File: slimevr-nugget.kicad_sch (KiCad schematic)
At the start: 56 parts, among them U1 nRF52840-QFXX, U3 XC6220B331MR, U4 LSM6DSV, U5 1532H, U6 QMC6309, U7 BQ24073RGT, Y1 32MHz

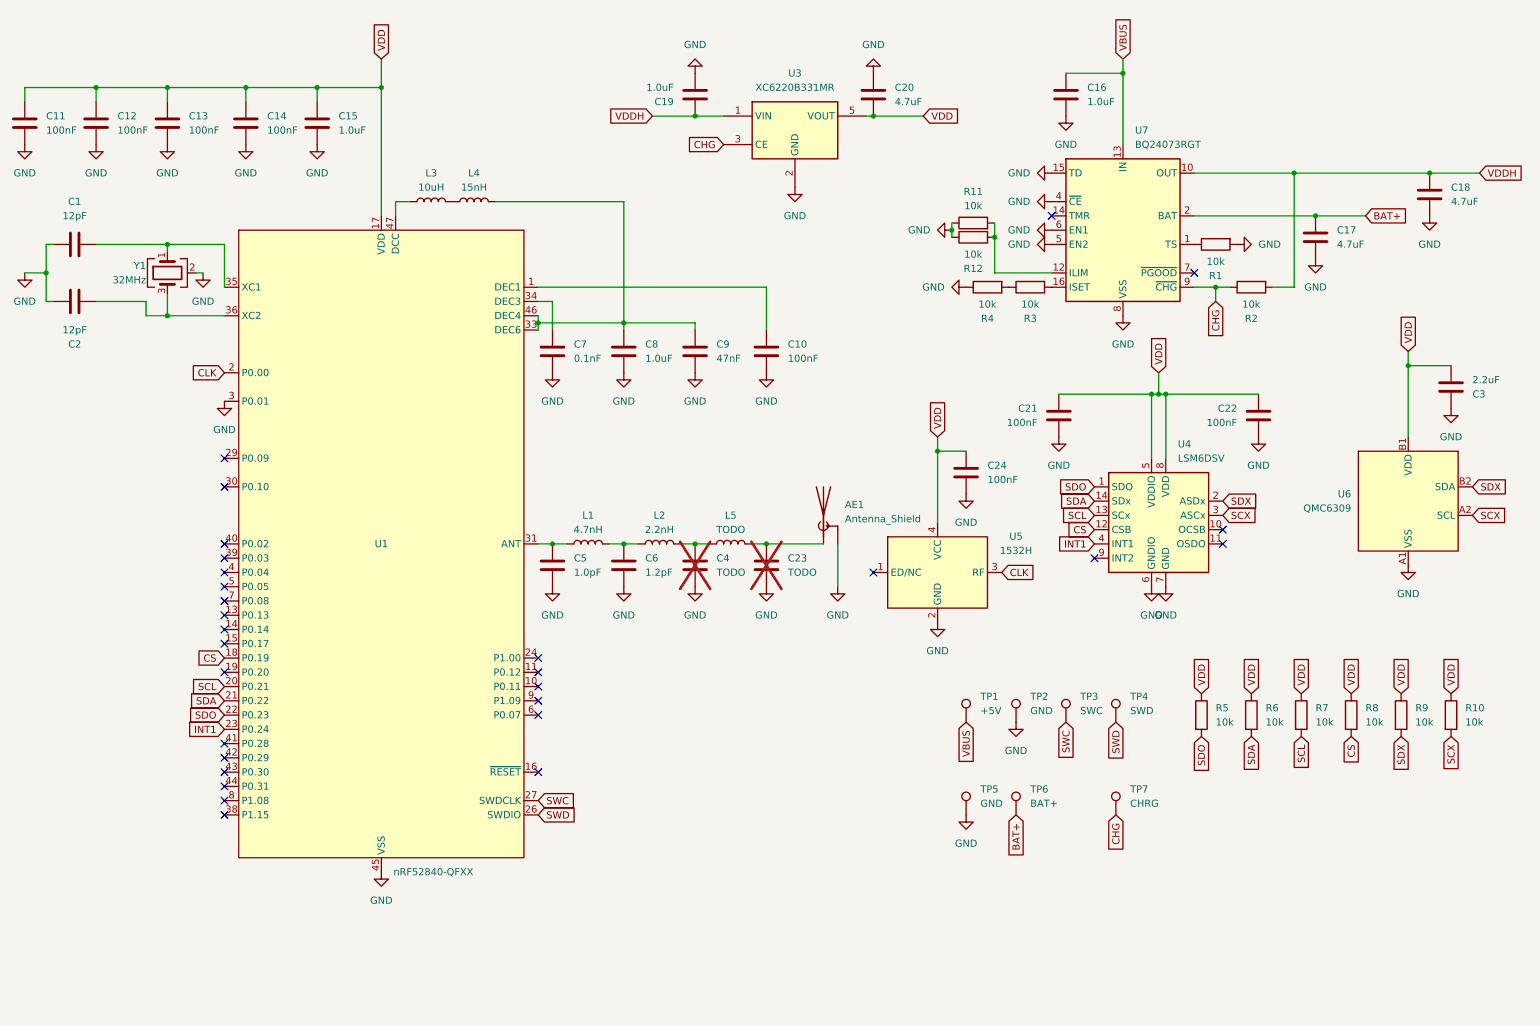
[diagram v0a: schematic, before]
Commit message: Final production version
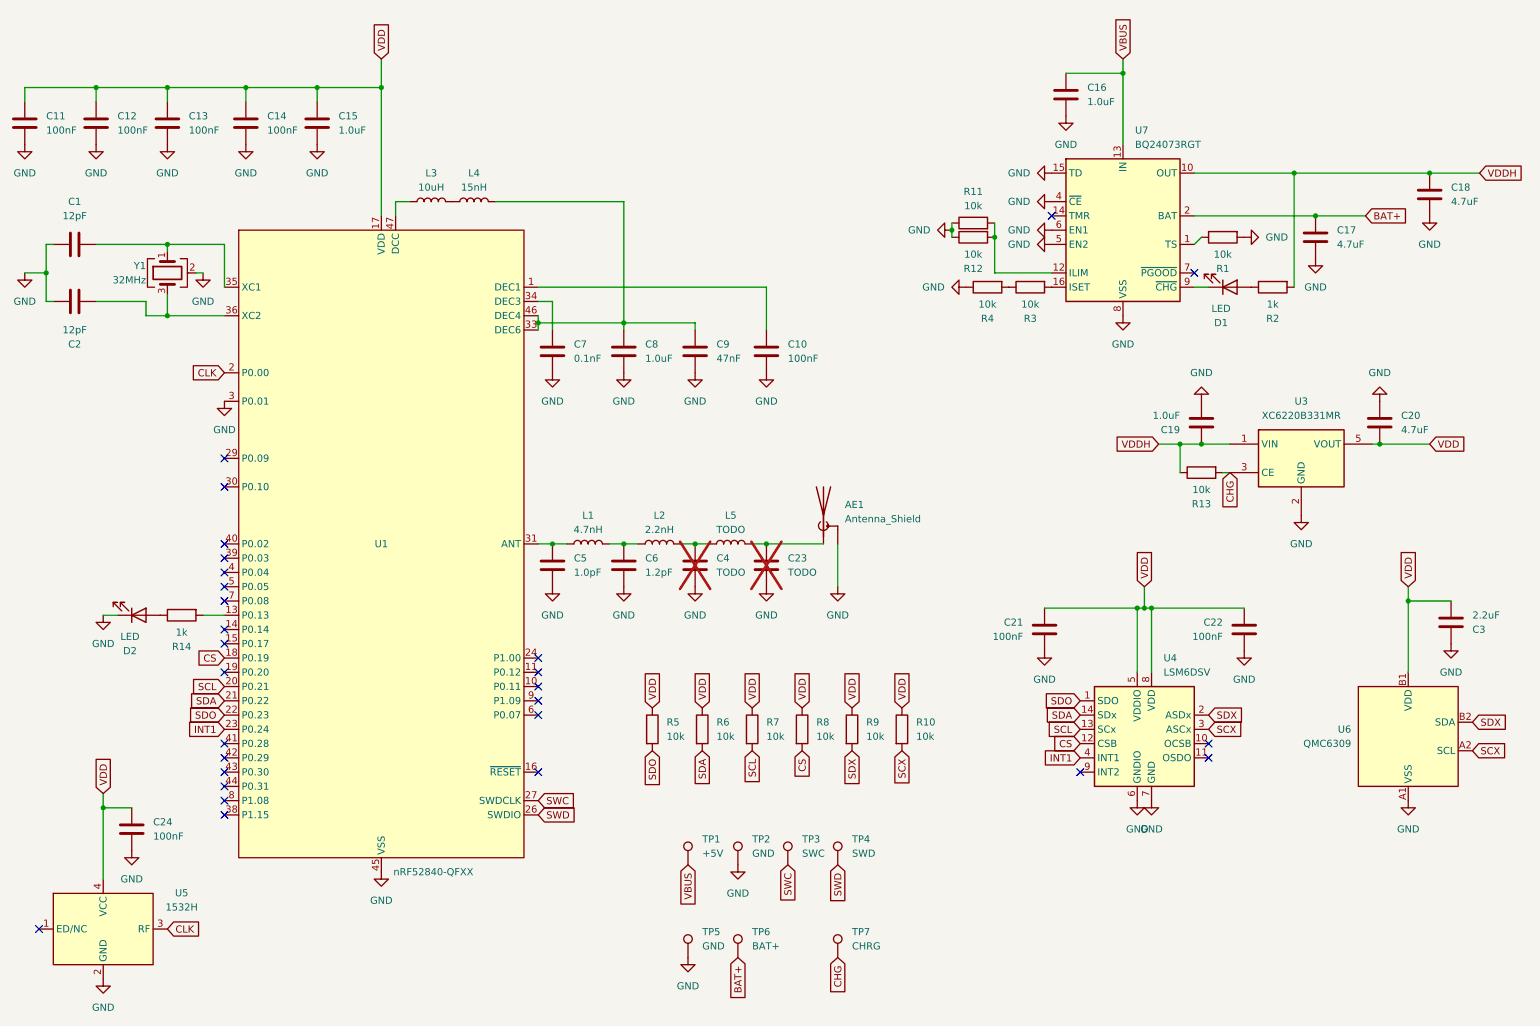
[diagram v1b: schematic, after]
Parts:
- added D1, D2: LED, LED_SMD:LED_0402_1005Metric, symbol Device:LED
- added R13: 10k, Resistor_SMD:R_0402_1005Metric, symbol Device:R
- added R14: 1k, Resistor_SMD:R_0402_1005Metric, symbol Device:R
- R2: value 10k -> 1k
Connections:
- net CHG: now also R13.2; no longer R2.1, U7.9 (~{CHG})
- net GND: now also D2.1 (K)
- net VDDH: now also R13.1
- net at U1.13 (P0.13): now also R14.2
- new net: D1.1 (K), U7.9 (~{CHG})
- new net: D2.2 (A), R14.1
- new net: D1.2 (A), R2.1
- no-connect marks 29 -> 28
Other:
- moved on the sheet: C19, C20, C21, C22, C24, C3, R1, R10, R2, R5, R6, R7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
